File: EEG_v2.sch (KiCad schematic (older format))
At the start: 11 parts, among them P1 CONN_2, P2 CONN_8, P3 USB_A, P4 CONN_8, P5 CONN_5X2, P6 CONN_2, P7 CONN_1, SW1 SWITCH_INV, SW2 RESET

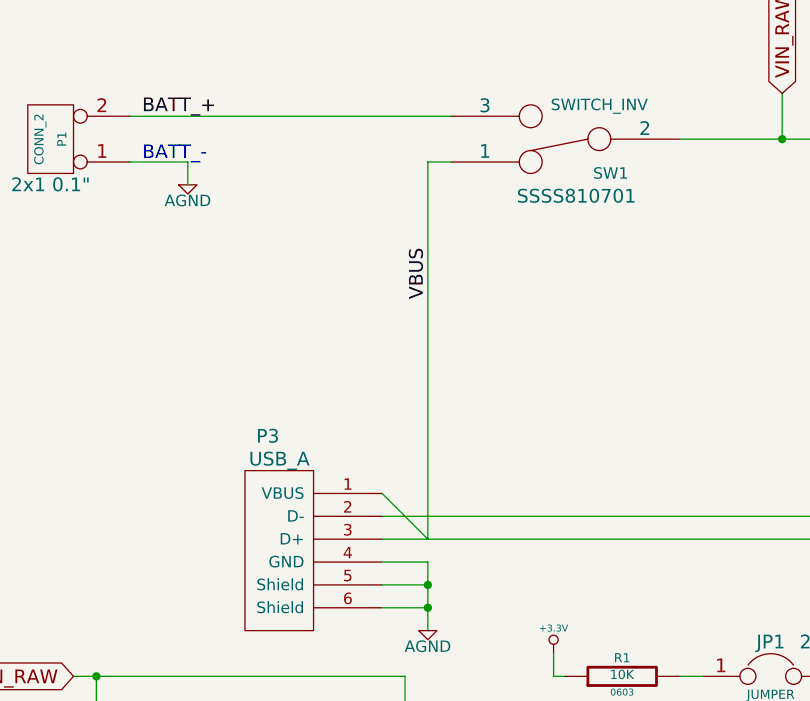
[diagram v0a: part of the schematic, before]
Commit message: Continue layout. Add fill zones.
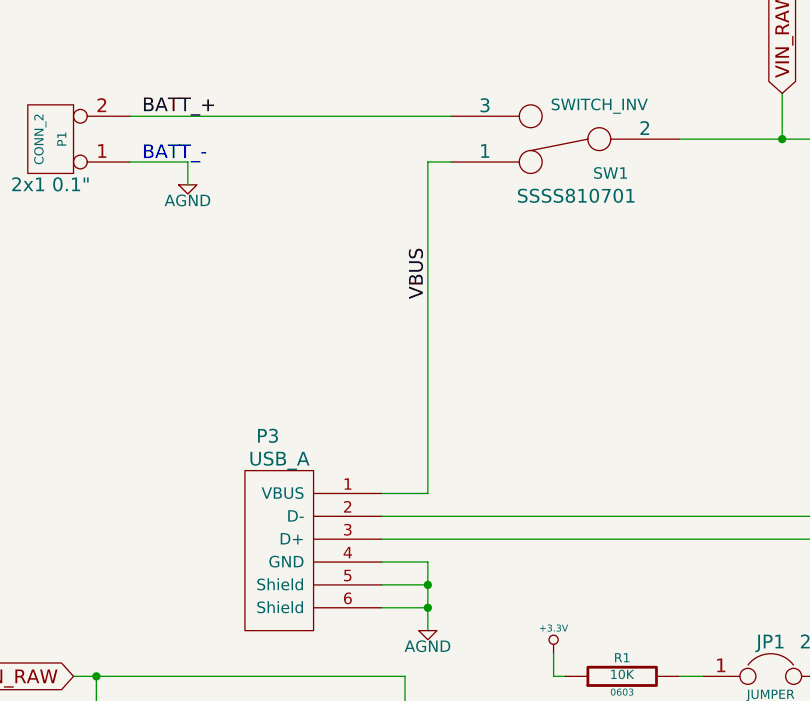
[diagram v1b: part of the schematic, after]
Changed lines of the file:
@@
 	4300 2700 4300 2900
 Wire Wire Line
-	2750 3000 2750 4650
+	2750 3000 2750 4450
 Wire Wire Line
 	4600 5250 4600 5850
@@
 	-1   0    0    1
 $EndComp
-Wire Wire Line
-	2750 4650 2550 4450
 Text Label 2750 3600 1    60   ~ 0
 VBUS
@@
 Connection ~ 4600 6500
 NoConn ~ 4700 5850
+Wire Wire Line
+	2750 4450 2550 4450
 $EndSCHEMATC
